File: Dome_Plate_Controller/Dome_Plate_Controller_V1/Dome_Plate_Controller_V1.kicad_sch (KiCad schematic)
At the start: 35 parts, among them J1 USB_B_Micro, J10 SERIAL_FU4, J11 SERIAL_FU3, J12 SERIAL_FU, J13 DB25_Female_MagTag, J14 DC-005-5A-2.0, J15 SERIAL_FU2, J2 DB25_Male_SlipRing, J3 12VOUT, J4 SERIAL_RS, J5 12OUT, J6 12VOUT, J7 5V OUT, J8 5V Out 2, J9 5V Out, SW1 SW_Push, U1 ESP32-WROOM-32D_16MB_, U2 CJ2301_S1, U3 ME6211C33M5G, U4 CH340C, U5 UMH3N, U6 D36V50F5-STEPDOWN

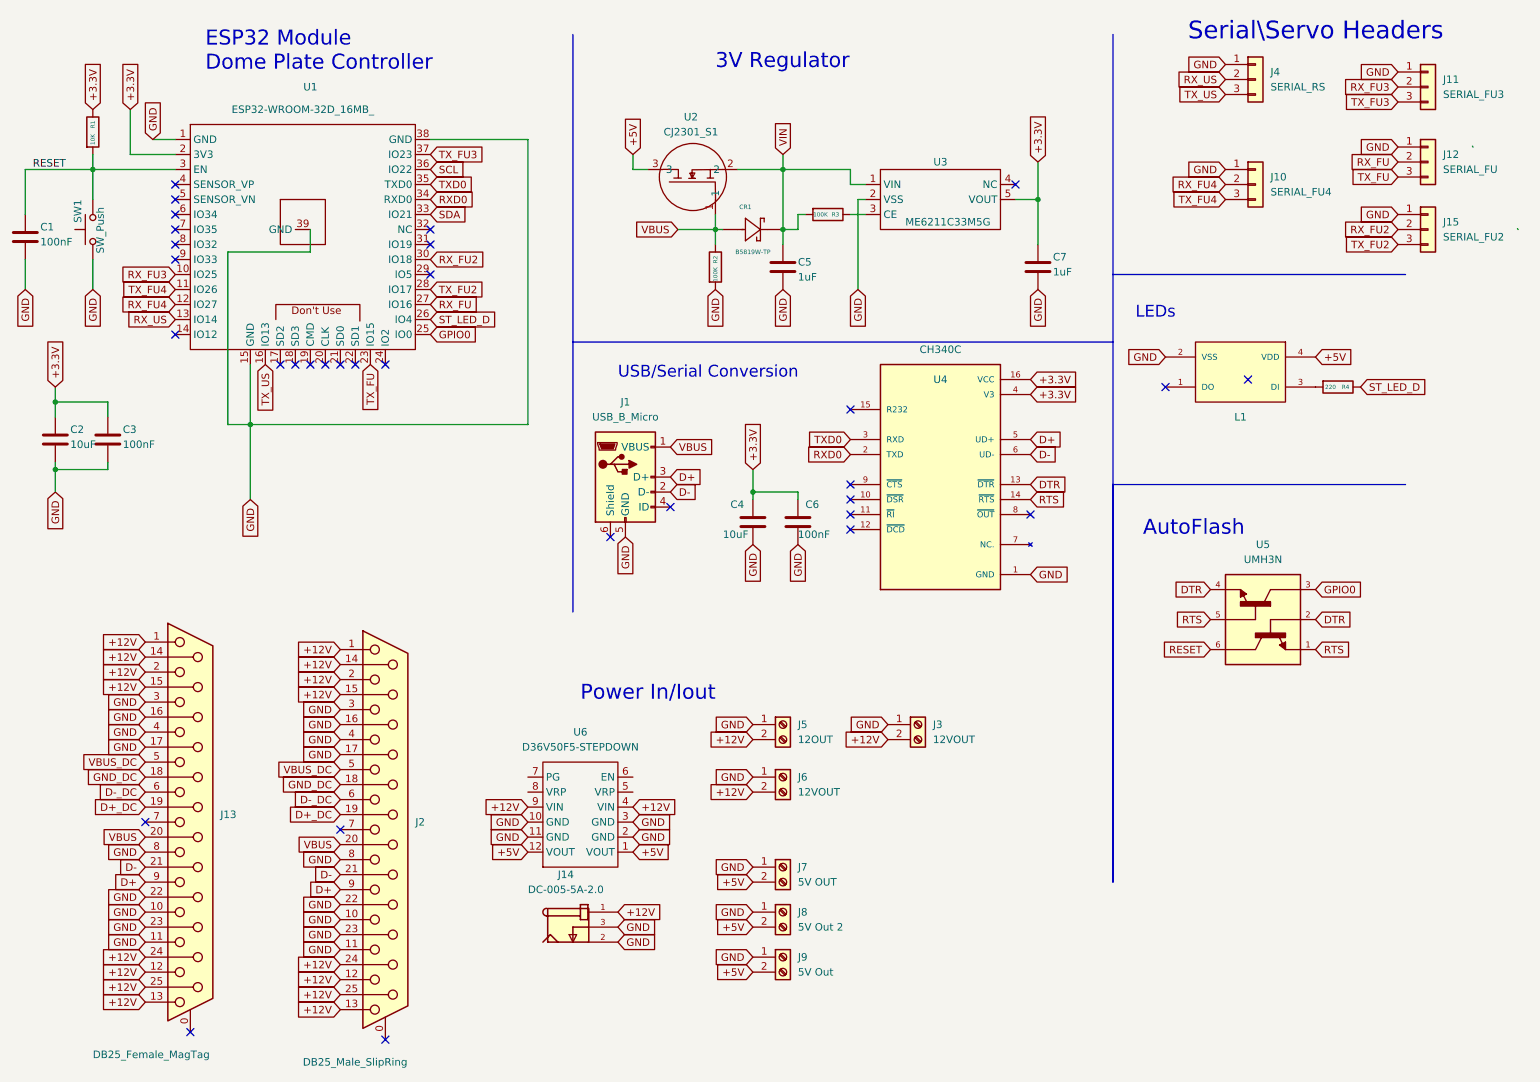
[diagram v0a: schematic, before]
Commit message: Added a lot since last check in
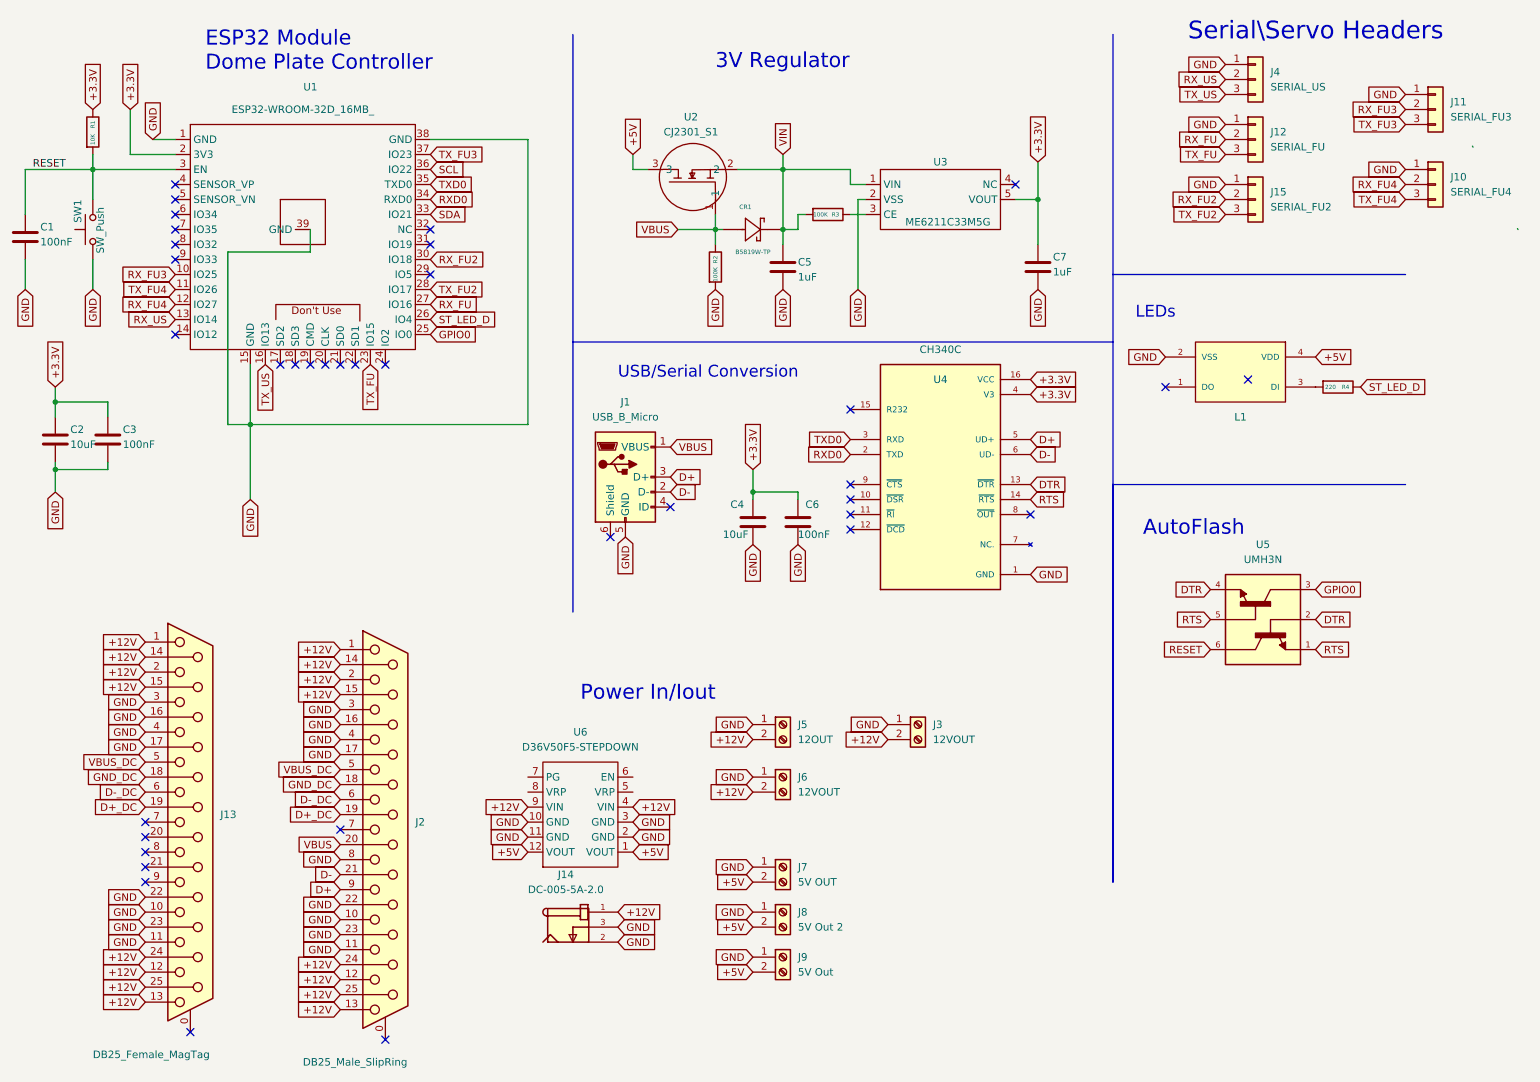
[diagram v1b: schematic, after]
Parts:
- J4: value SERIAL_RS -> SERIAL_US
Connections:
- net D+: no longer J13.9
- net D-: no longer J13.21 (P21)
- net GND: no longer J13.8
- net VBUS: no longer J13.20 (P20)
- no-connect marks 32 -> 36
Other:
- moved on the sheet: J10, J11, J12, J15
